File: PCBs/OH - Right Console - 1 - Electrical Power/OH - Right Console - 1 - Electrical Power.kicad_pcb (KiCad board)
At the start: 2 copper layers, 59.9 x 33.3 mm, 15 parts, among them J1 Switch Inputs, J2 Batt U Volts In, J3 Batt E Volts In, J4 Batt U Volts Out, J5 Batt U Volts Out, SW1 EXT PWR, SW2 R GEN, SW3 L GEN

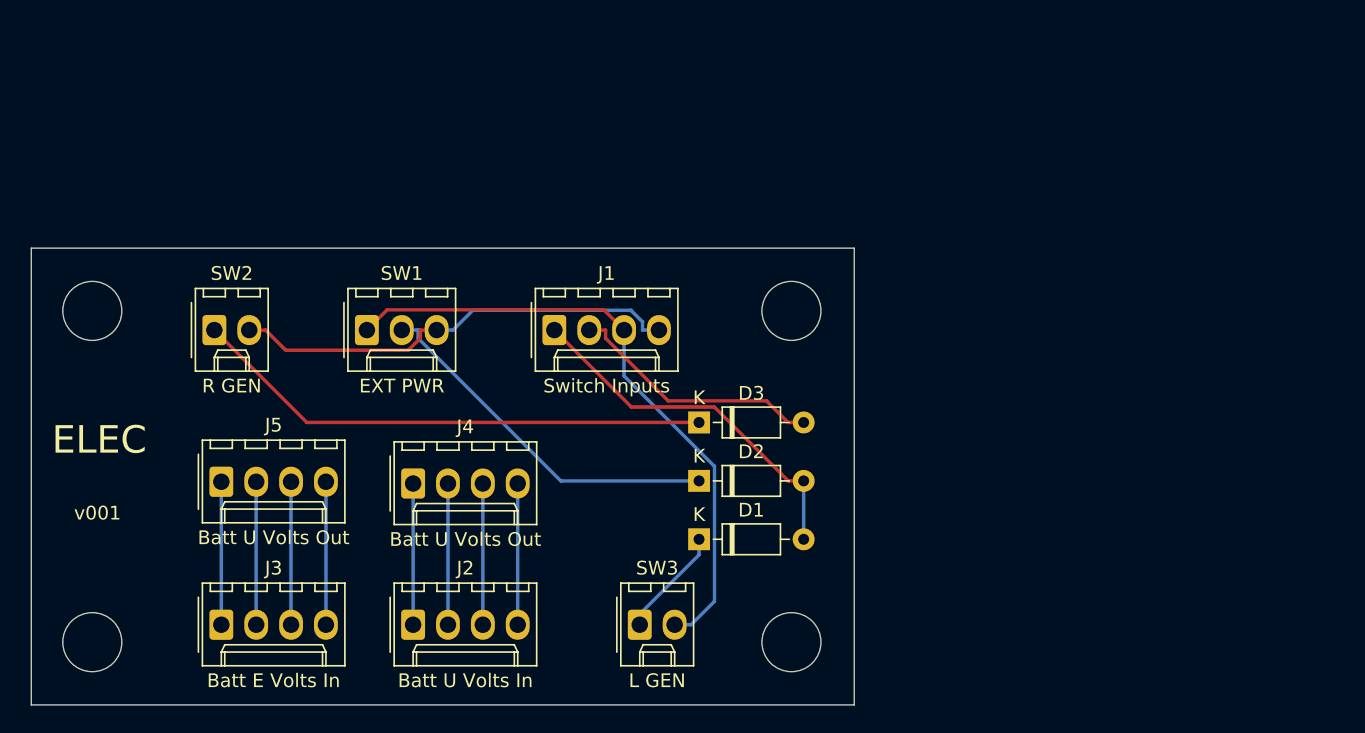
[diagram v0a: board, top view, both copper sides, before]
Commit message: Elect Power Done
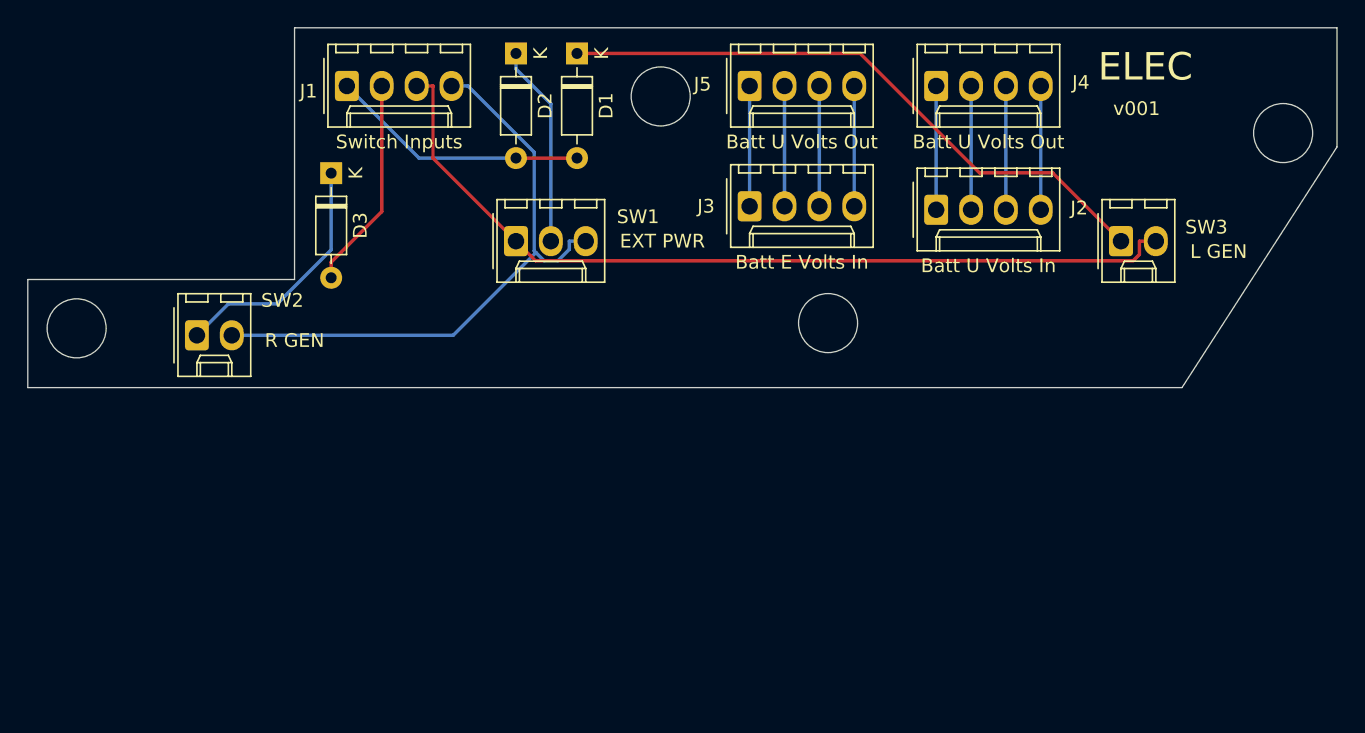
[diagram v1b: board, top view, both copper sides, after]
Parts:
- moved H1 53.6 mm to (138.9, 99.3)
- moved H4 51.6 mm to (172.1, 85.5)
- moved J3 49.1 mm to (133.2, 90.8)
- moved J2 48.6 mm to (146.8, 91.1)
- moved J5 48.1 mm to (133.2, 82.0)
- moved J4 47.9 mm to (146.8, 82.0)
- moved SW3 44.8 mm to (160.3, 93.3)
- moved D1 36.5 mm to (120.7, 79.7), turned to 270 degrees
- moved D2 33.9 mm to (116.2, 79.7), turned to 270 degrees
- moved D3 32.4 mm to (102.7, 88.4), turned to 270 degrees
- moved J1 23.3 mm to (103.9, 82.0)
- moved H2 22.9 mm to (84.2, 99.7)
- moved H3 18.3 mm to (126.7, 82.8)
- moved SW1 12.6 mm to (116.2, 93.3)
- moved SW2 1.33 mm to (93.0, 100.2)
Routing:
- net Net-(D1-Pad1): track 8.01 -> 45.3 mm
- net Net-(D3-Pad1): track 38.1 -> 17.9 mm
- net /Row1: track 46.0 -> 63.4 mm
- net /Row2: track 33.0 -> 44.9 mm
- net Net-(D2-Pad1): track 26.6 -> 14.7 mm
- net Net-(D1-Pad2): track 27.0 -> 18.9 mm
- net Net-(D3-Pad2): track 18.8 -> 15.5 mm
- net Net-(J3-Pad4): track 10.4 -> 8.76 mm
- net Net-(J3-Pad3): track 10.4 -> 8.76 mm
- net Net-(J3-Pad2): track 10.4 -> 8.76 mm
- net Net-(J3-Pad1): track 10.4 -> 8.76 mm
- net Net-(J2-Pad4): track 10.3 -> 9.02 mm
- net Net-(J2-Pad3): track 10.3 -> 9.02 mm
- net Net-(J2-Pad2): track 10.3 -> 9.02 mm
- net Net-(J2-Pad1): track 10.3 -> 9.02 mm
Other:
- board size 59.9 x 33.3 mm -> 95.4 x 26.2 mm
